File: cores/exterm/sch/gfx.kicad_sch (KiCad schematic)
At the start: 23 parts

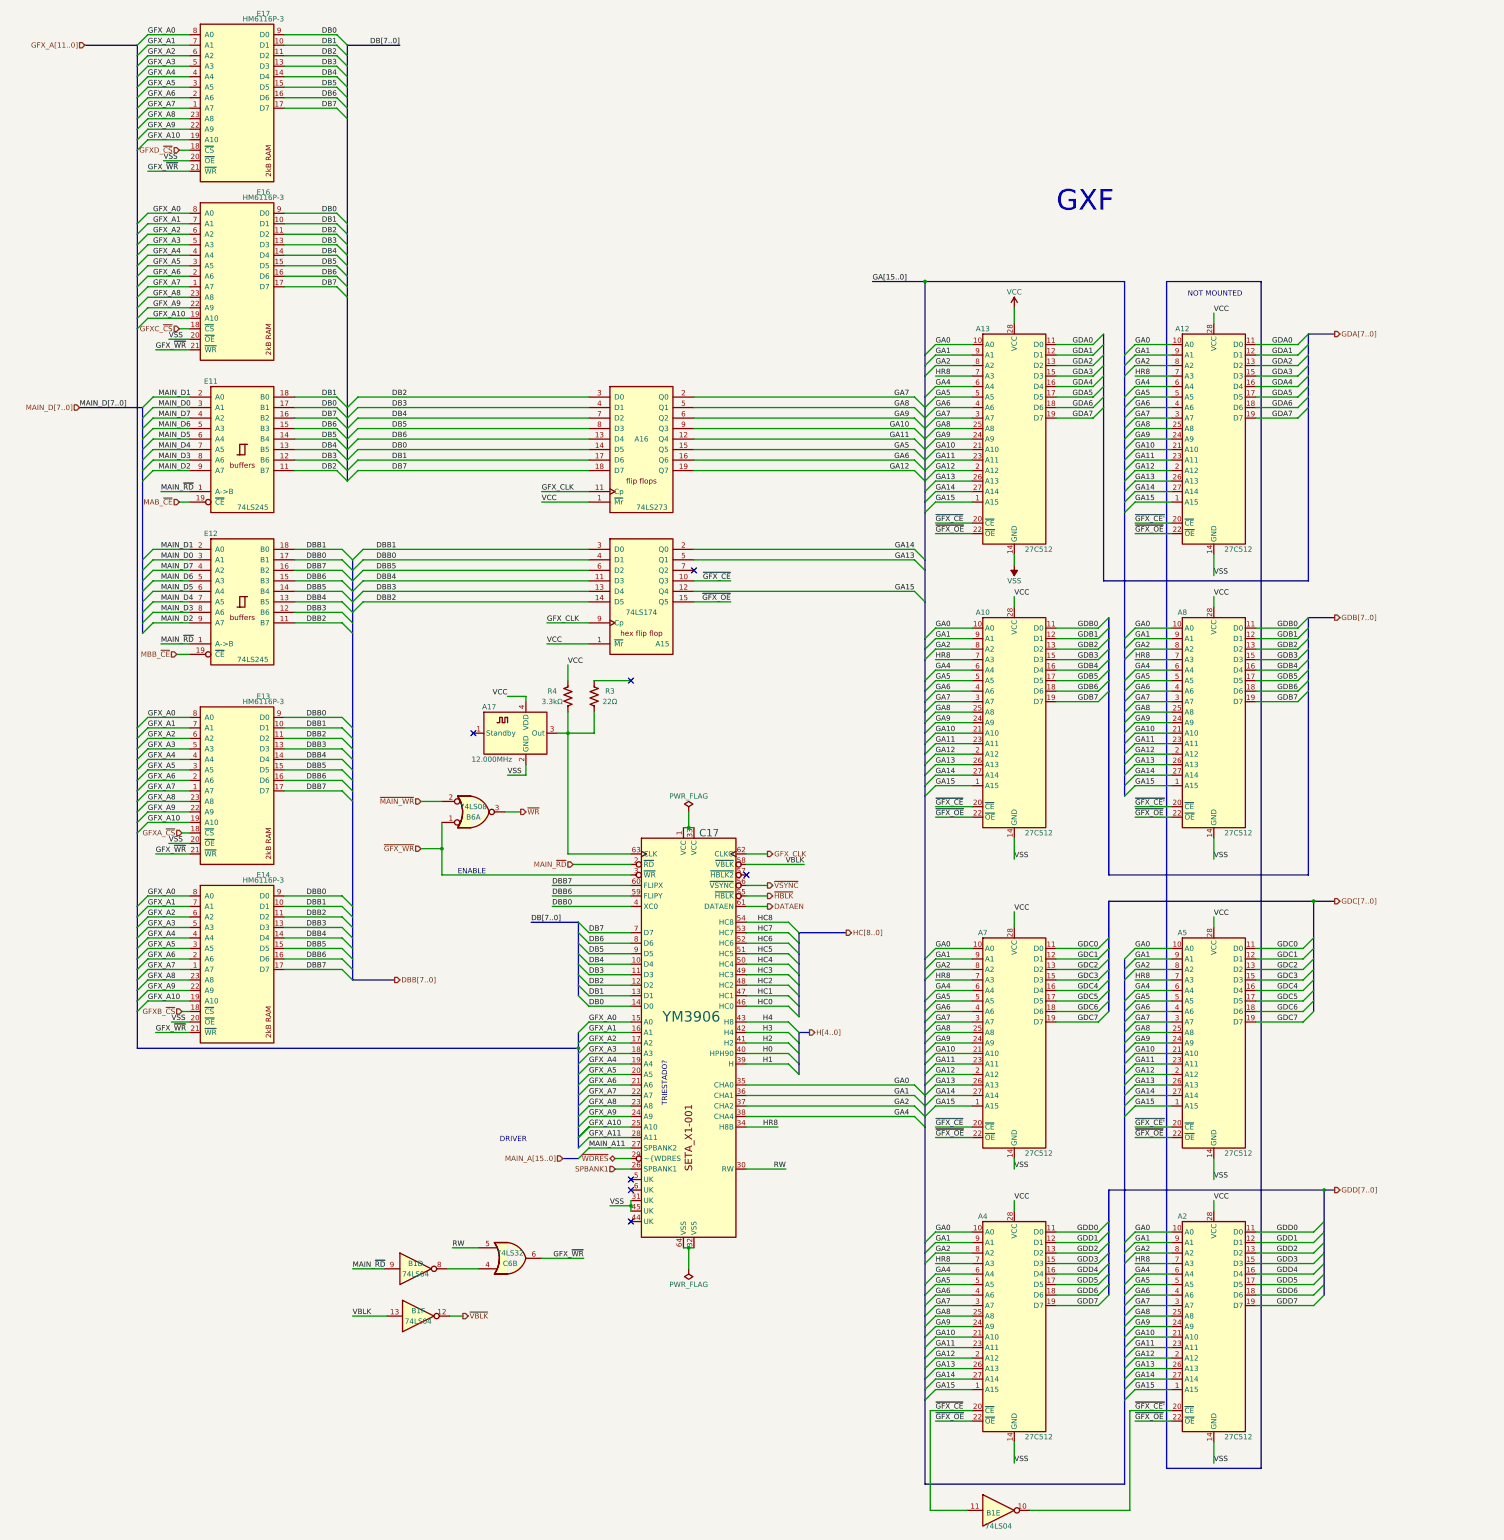
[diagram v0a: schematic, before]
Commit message: issues_solved_#21
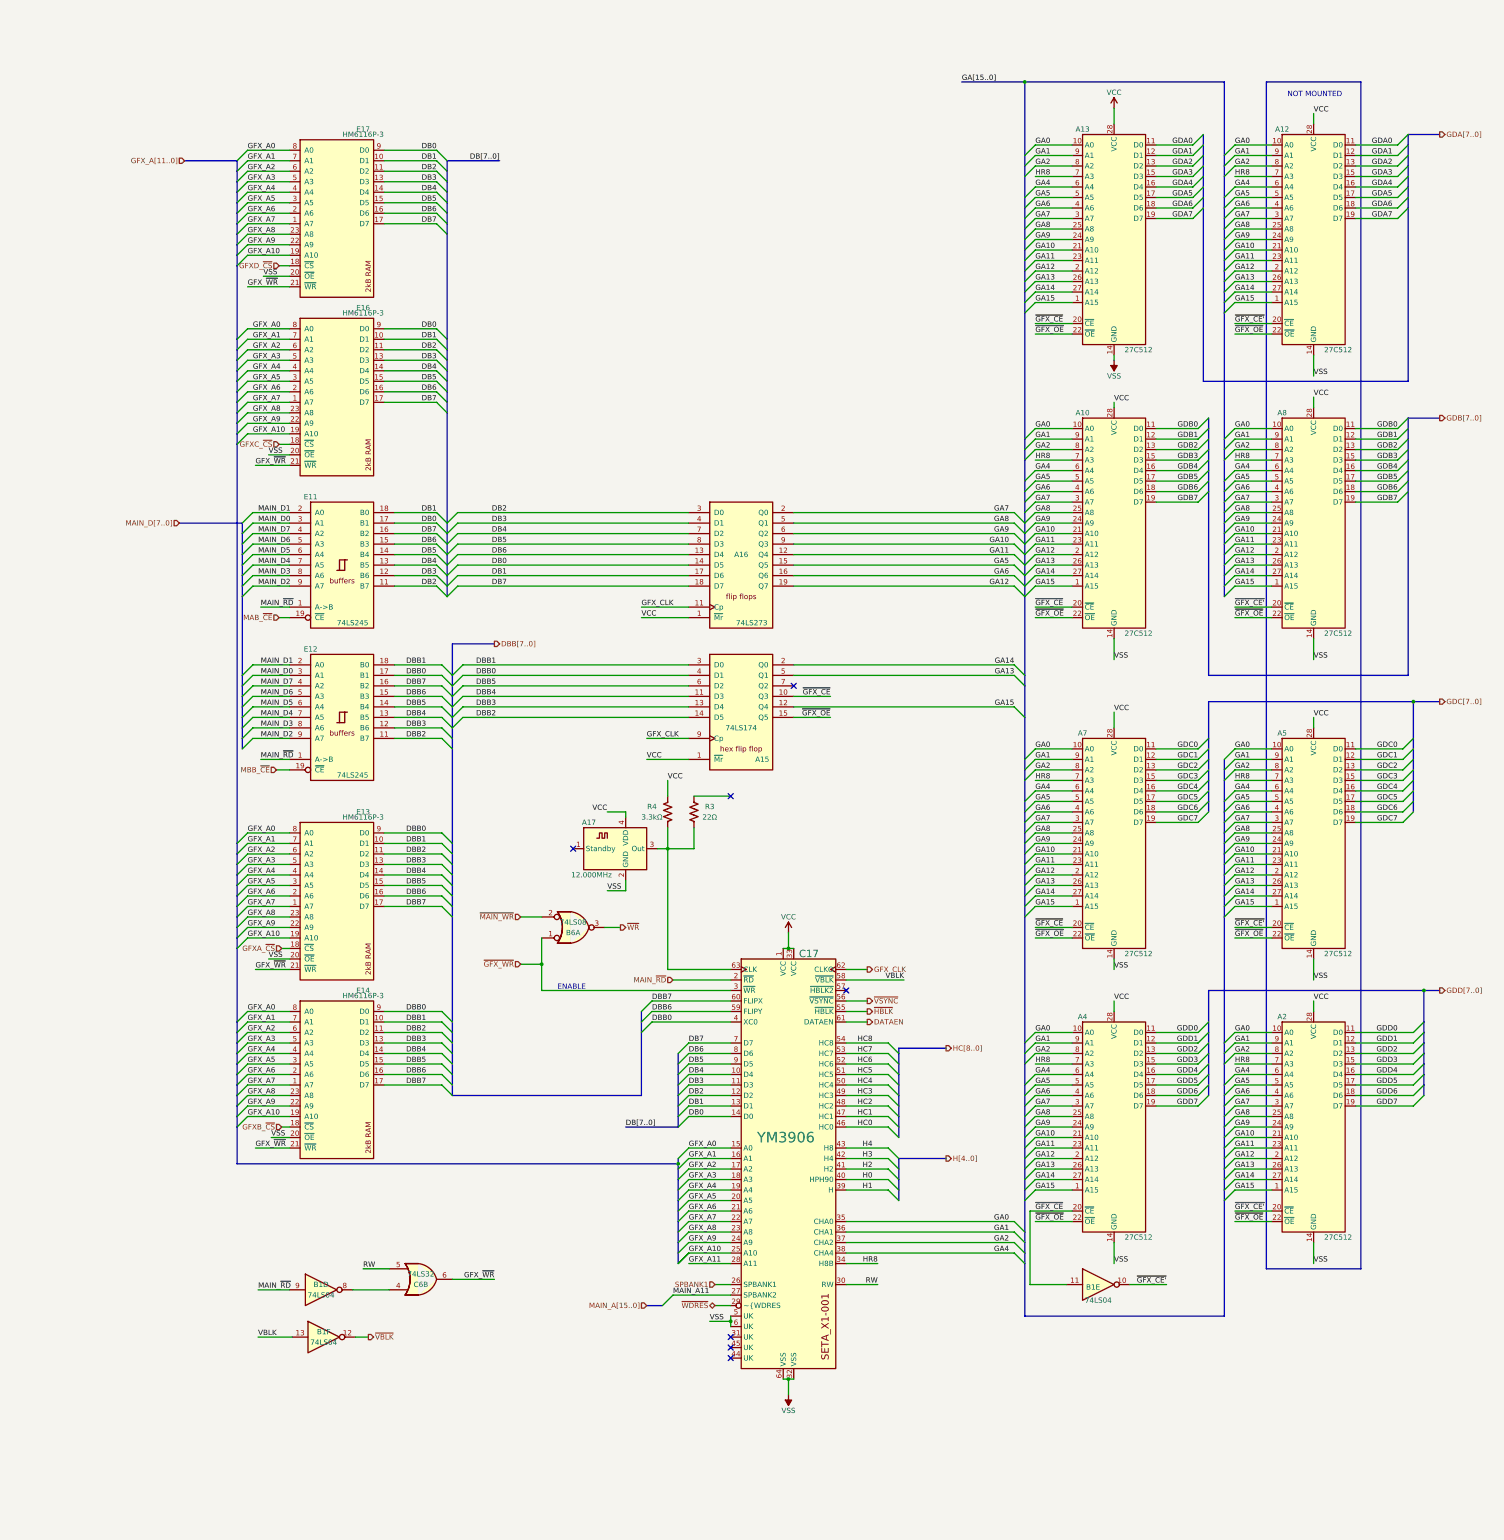
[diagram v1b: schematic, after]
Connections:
- net VCC: now also C17.1 (VCC), C17.33 (VCC)
- net VSS: now also C17.32 (VSS), C17.5 (UK), C17.6 (UK), C17.64 (VSS); no longer C17.31 (UK), C17.45 (UK)
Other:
- note removed: "DRIVER"
- note removed: "GXF"
- note removed: "TRIESTADO?"
- moved on the sheet: A10, A12, A13, A15, A16, A17, A2, A4, A5, A7, A8, B1D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
